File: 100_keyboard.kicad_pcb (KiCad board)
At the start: 2 copper layers, 92.7 x 49.5 mm, 22 parts, among them SW1 SW_Push, U1 MIC5219-3.3YM5, U2 STM32F072RBTx

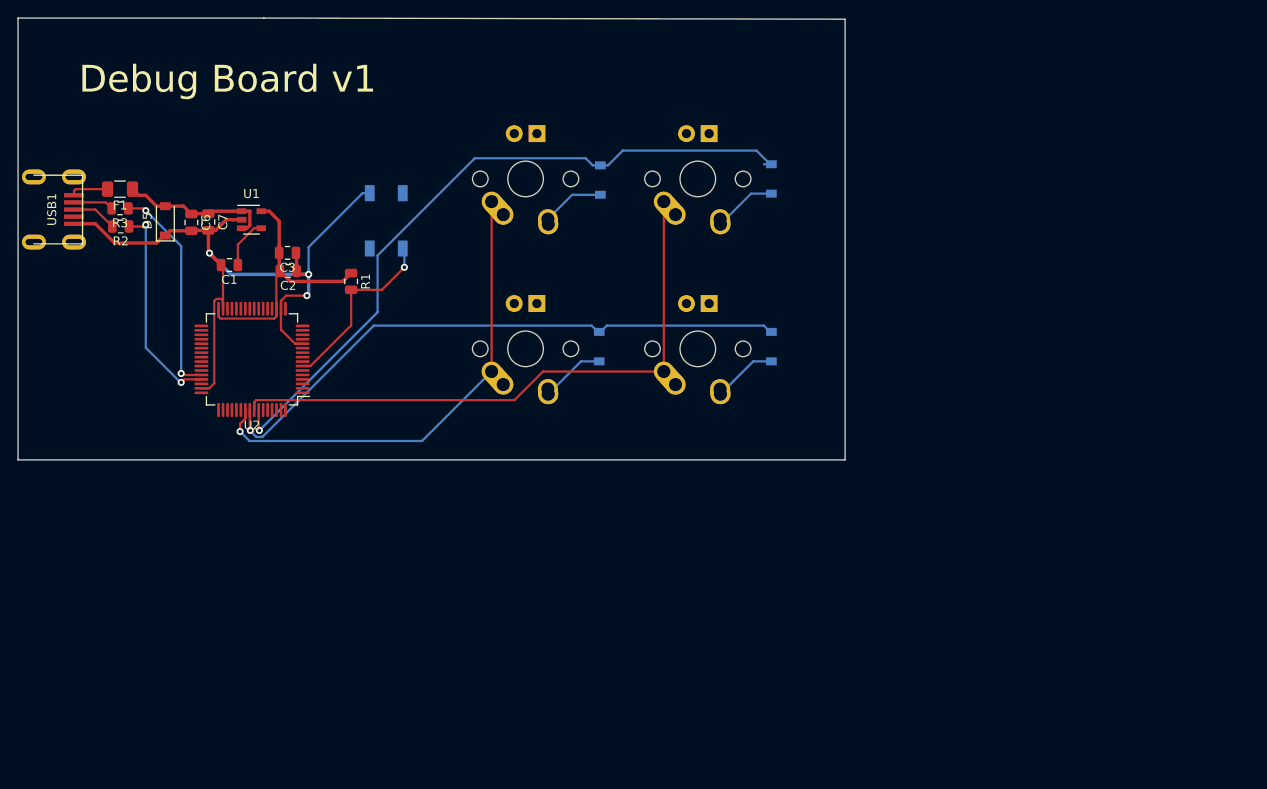
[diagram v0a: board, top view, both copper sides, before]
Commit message: Debug board v0.2
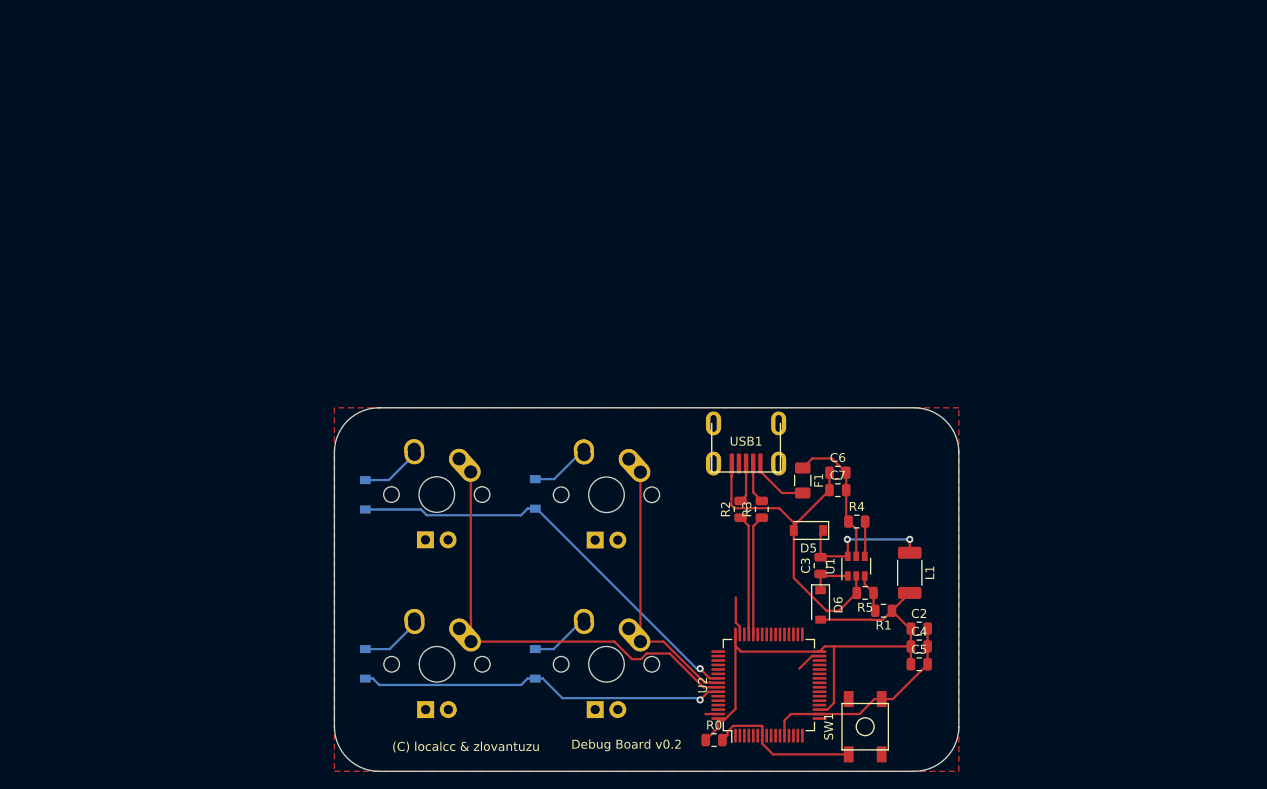
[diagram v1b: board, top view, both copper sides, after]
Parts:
- removed C1: 470pF, Capacitor_SMD:C_0805_2012Metric
- added C4: 0.1uF, Capacitor_SMD:C_0805_2012Metric, F.Cu at (143.1, 106.0)
- added C5: 0.1uF, Capacitor_SMD:C_0805_2012Metric, F.Cu at (143.1, 108.0)
- added D6: 1N4148, Diode_SMD:D_SOD-123, F.Cu at (132.0, 101.3)
- added L1: 47uH/1.66A, Inductor_SMD:L_2010_5025Metric, F.Cu at (142.0, 97.8)
- added R0: 10k, Resistor_SMD:R_0805_2012Metric, F.Cu at (120.1, 116.5)
- added R4: 100kOhm, Resistor_SMD:R_0805_2012Metric, F.Cu at (136.1, 92.0)
- added R5: 16.2kOhm, Resistor_SMD:R_0805_2012Metric, F.Cu at (137.0, 100.0)
- C2: value 0.1uF -> 22uF 6.3V
- C3: value 0.1uF -> 22nF
- D5: value D_Small -> D_Schottky
- R1: value 10k -> 50kOhm
- SW1: moved to F.Cu
- U1: value MIC5219-3.3YM5 -> mp2359; footprint Package_TO_SOT_SMD:SOT-23-5 -> Package_TO_SOT_SMD:SOT-23-6
- moved USB1 83.4 mm to (123.7, 81.0), turned to 270 degrees
- moved F1 83.2 mm to (130.0, 87.4), turned to 270 degrees
- moved C2 81.3 mm to (143.1, 104.0), turned to 0 degrees
- moved D5 80.0 mm to (130.7, 93.0), turned to 180 degrees
- moved R3 79.5 mm to (125.4, 90.6), turned to 90 degrees
- moved U1 78.1 mm to (136.0, 97.0), turned to 90 degrees
- moved SW1 78.1 mm to (137.0, 115.0)
- moved C6 77.7 mm to (133.9, 86.5), turned to 0 degrees
- moved C7 76.7 mm to (133.9, 88.5), turned to 0 degrees
- moved R2 76.4 mm to (123.0, 90.6), turned to 90 degrees
- moved R1 70.2 mm to (139.1, 102.0), turned to 180 degrees
- moved C3 69.3 mm to (132.0, 96.9), turned to 90 degrees
- moved U2 68.5 mm to (126.2, 110.3), turned to 90 degrees
- moved D4 60.5 mm to (100.0, 108.0), turned to 90 degrees
- moved D3 60.3 mm to (81.0, 108.0), turned to 90 degrees
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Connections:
- C2 pad 1: GND -> 3.3V
- C2 pad 2: 3.3V -> GND
- C3 pad 1: GND -> Net-(C3-Pad1)
- C3 pad 2: 3.3V -> Net-(C3-Pad2)
- C6 pad 1: +5V -> GND
- C6 pad 2: GND -> +5V
- C7 pad 1: +5V -> GND
- C7 pad 2: GND -> +5V
- D5 pad 1: GND -> Net-(C3-Pad2)
- D5 pad 2: +5V -> GND
- R1 pad 2: NRST -> Net-(R1-Pad2)
- U1 pad 1: +5V -> Net-(C3-Pad1)
- U1 pad 3: +5V -> Net-(R1-Pad2)
- U1 pad 5: 3.3V -> +5V
- U2 pad 55: COL0 -> ROW0
- U2 pad 56: ROW0 -> COL1
- U2 pad 57: COL1 -> COL0
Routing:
- net COL1: track 67.3 -> 29.6 mm
- net ROW1: track 78.6 -> 41.5 mm
- net 3.3V: track 30.0 -> 60.6 mm
- net ROW0: track 67.1 -> 48.0 mm
- net Net-(C3-Pad2): track 0.00 -> 16.6 mm, vias 0 -> 2
- net GND: track 83.2 -> 71.2 mm, vias 3 -> 0
- net Net-(R3-Pad1): track 24.3 -> 13.5 mm, vias 2 -> 0
- net Net-(R2-Pad1): track 23.7 -> 13.5 mm, vias 2 -> 0
- net Net-(C3-Pad1): track 0.00 -> 4.97 mm
- net Net-(R1-Pad2): track 0.00 -> 4.39 mm
- net COL0: track 53.8 -> 49.4 mm, vias 1 -> 0
- net NRST: track 20.5 -> 17.5 mm, vias 1 -> 0
- net VCC: track 4.33 -> 6.63 mm
- net Net-(R4-Pad2): track 5.68 -> 3.92 mm
- net +5V: track 17.1 -> 15.8 mm
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- added copper zone on F.Cu, net GND
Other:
- board size 92.7 x 49.5 mm -> 70 x 40.8 mm
- board text added: "Debug Board v0.2"
- board text added: "GitHub: https://github.com/localcc https://github.com/zlovantuzu"
- board text removed: "Debug Board v1"
- board text removed: "Github: https://github.com/localcc https://github.com/zlovantuzu"

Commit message: Debug Board v0.3
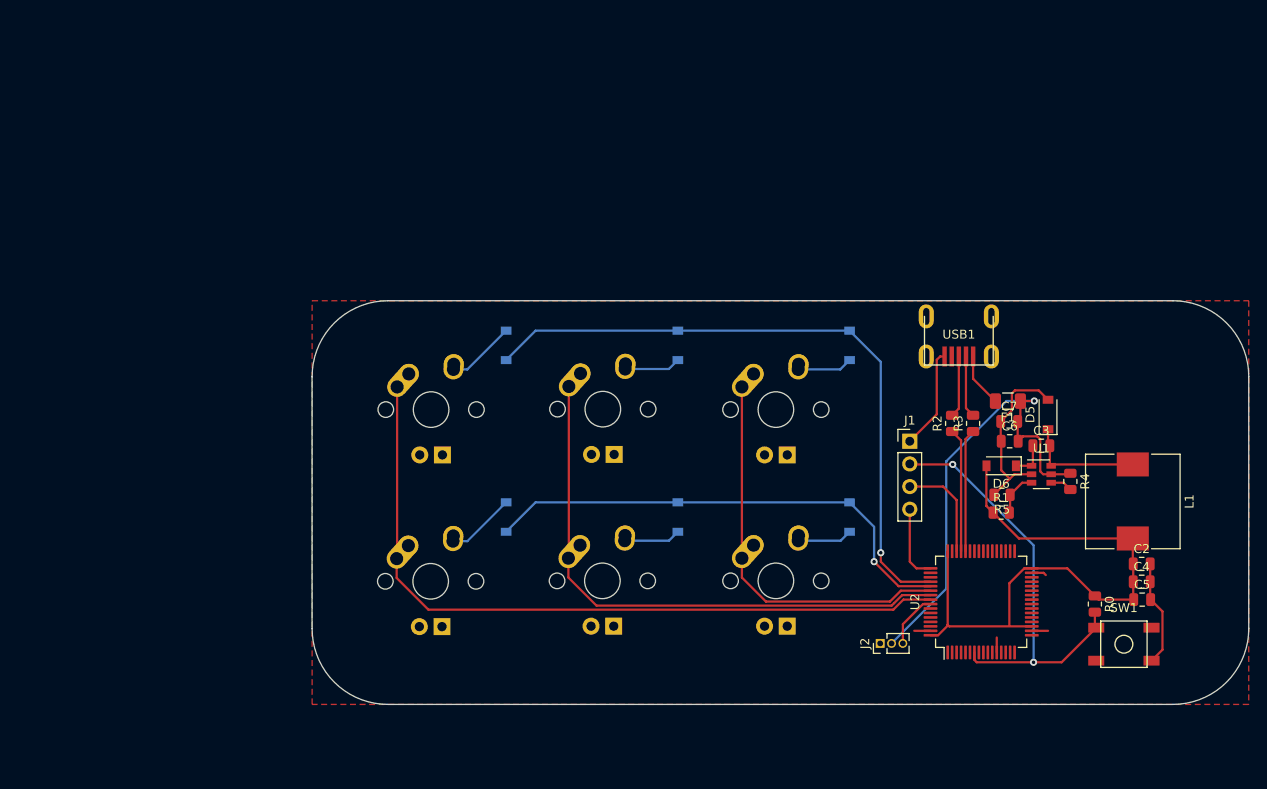
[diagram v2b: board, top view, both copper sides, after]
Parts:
- added D7: D_Small, Diode_SMD:D_SOD-123, B.Cu at (135.2, 72.2)
- added D8: D_Small, Diode_SMD:D_SOD-123, B.Cu at (135.2, 91.5)
- added J1: Conn_01x04, Connector_PinHeader_2.54mm:PinHeader_1x04_P2.54mm_Vertical, F.Cu at (142.0, 83.0)
- added J2: Conn_01x03, Connector_PinHeader_1.27mm:PinHeader_1x03_P1.27mm_Vertical, F.Cu at (138.7, 105.7)
- added MX5: MX-NoLED, MX_Alps_Hybrid:MX-1U, F.Cu at (127.0, 79.5)
- added MX6: MX-NoLED, MX_Alps_Hybrid:MX-1U, F.Cu at (127.0, 98.7)
- L1: footprint Inductor_SMD:L_2010_5025Metric -> Inductor_SMD:L_10.4x10.4_H4.8
- MX1, MX2, MX3, MX4: moved to F.Cu
- moved R0 45.3 mm to (162.8, 101.2), turned to 270 degrees
- moved SW1 30.4 mm to (166.0, 105.8), turned to 180 degrees
- moved D5 29.8 mm to (157.5, 80.0), turned to 90 degrees
- moved C3 28.2 mm to (156.8, 83.5), turned to 0 degrees
- moved USB1 26.7 mm to (147.5, 69.0)
- moved L1 26.2 mm to (167.0, 89.8)
- moved C5 26.0 mm to (168.1, 100.8)
- moved C2 26.0 mm to (168.0, 96.8)
- moved C4 26.0 mm to (168.0, 98.8)
- moved R2 25.6 mm to (146.8, 81.0)
- moved R3 25.6 mm to (149.1, 81.0)
- moved D6 25.6 mm to (152.2, 85.8), turned to 180 degrees
- moved U2 25.6 mm to (150.0, 101.0)
- moved F1 24.7 mm to (153.0, 78.5), turned to 180 degrees
- moved R4 24.4 mm to (160.0, 87.5), turned to 270 degrees
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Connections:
- U2 pad 46: Net-(U2-Pad46) -> SWDIO
- U2 pad 49: Net-(U2-Pad49) -> SWDCLK
- U2 pad 52: Net-(U2-Pad52) -> ROW0
- U2 pad 53: Net-(U2-Pad53) -> ROW1
- U2 pad 54: Net-(U2-Pad54) -> COL2
- U2 pad 55: ROW0 -> COL1
- U2 pad 56: COL1 -> COL0
- U2 pad 57: COL0 -> LED_SPI
- U2 pad 58: ROW1 -> Net-(U2-Pad58)
- U2 pad 60: Net-(U2-Pad60) -> GND
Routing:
- net COL2: track 0.00 -> 44.1 mm
- net +5V: track 15.8 -> 51.8 mm, vias 0 -> 1
- net COL1: track 29.6 -> 63.8 mm
- net COL0: track 49.4 -> 83.2 mm
- net NRST: track 17.5 -> 48.8 mm, vias 0 -> 2
- net ROW0: track 48.0 -> 73.7 mm
- net GND: track 71.2 -> 50.7 mm
- net ROW1: track 41.5 -> 55.1 mm
- net SWDIO: track 0.00 -> 11.6 mm
- net 3.3V: track 60.6 -> 70.3 mm
- net SWDCLK: track 0.00 -> 8.52 mm
- net Net-(D7-Pad2): track 0.00 -> 6.19 mm
- net LED_SPI: track 0.00 -> 6.19 mm
- net Net-(D8-Pad2): track 0.00 -> 6.17 mm
- net Net-(C3-Pad2): track 16.6 -> 13.5 mm, vias 2 -> 0
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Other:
- board size 70 x 40.8 mm -> 105 x 45.2 mm
- board text removed: "(C) localcc & zlovantuzu"
- board text removed: "Debug Board v0.2"
- board text removed: "GitHub: https://github.com/localcc https://github.com/zlovantuzu"
